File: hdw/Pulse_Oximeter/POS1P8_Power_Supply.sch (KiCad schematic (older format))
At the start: 0 parts

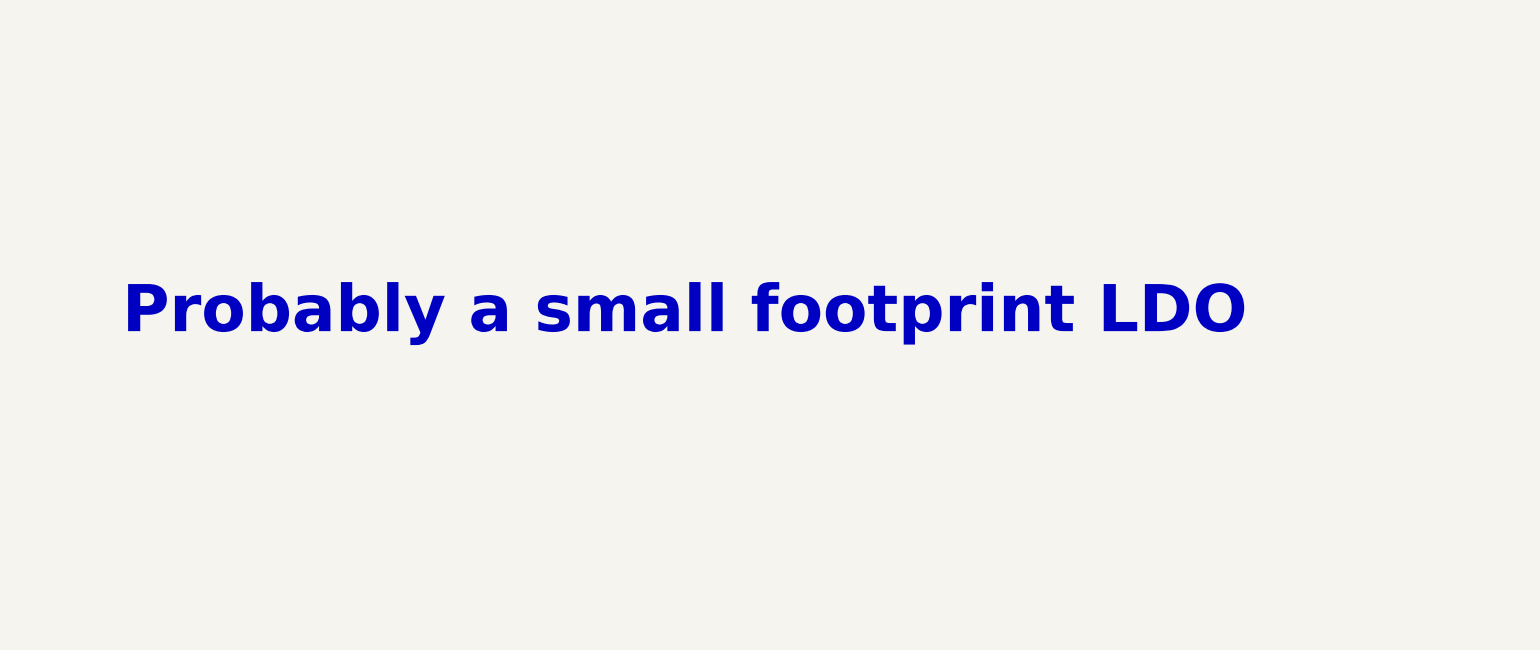
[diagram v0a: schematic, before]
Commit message: Continued schematic development
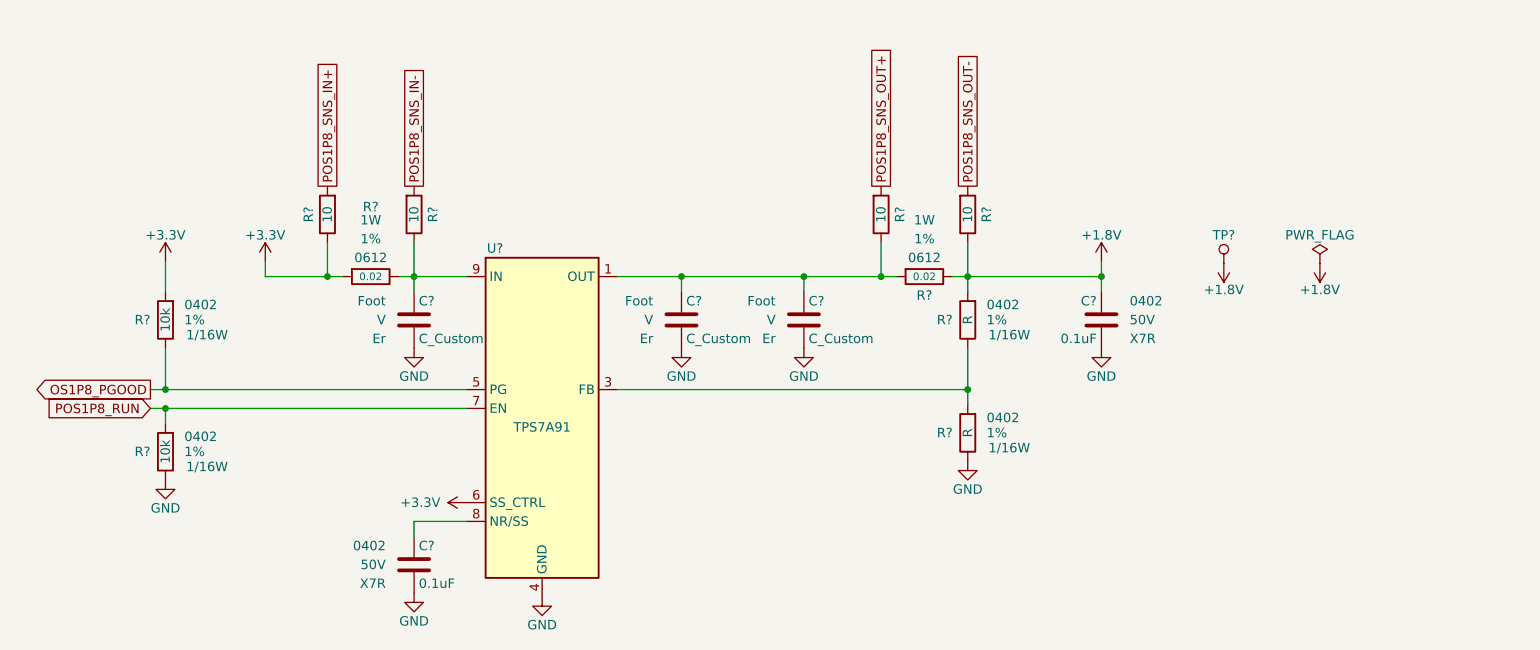
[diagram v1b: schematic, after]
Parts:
- added C? (x2): 0.1uF, Capacitors_SMD:C_0402, symbol Custom_Library:C_Custom
- added C? (x3): C_Custom, symbol Custom_Library:C_Custom
- added R? (x2): 10k, Resistors_SMD:R_0402, symbol Custom_Library:R_Custom
- added R? (x2): 0.02, Resistors_SMD:R_0612, symbol Custom_Library:R_Custom
- added R? (x4): 10, Resistors_SMD:R_0603, symbol Custom_Library:R_Custom
- added R? (x2): R, Resistors_SMD:R_0402, symbol Custom_Library:R_Custom
- added TP?: TP, Custom Footprints Library:Test_Point, symbol Custom_Library:TP
- added U?: TPS7A91, Package_DFN_QFN:Texas_S-PDSO-N10_EP1.2x2mm, symbol Custom_Library:TPS7A91
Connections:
- new net: C?.1, U?.8 (NR/SS)
- new net: C?.1, C?.1, R?.1, R?.2, U?.1 (OUT), U?.2 (OUT)
- new net: C?.1, R?.2, R?.2, U?.10 (IN), U?.9 (IN)
- new net: R?.1, R?.2, U?.3 (FB)
- new net +1.8V: C?.1, R?.1, R?.2, R?.2, TP?.1 (TP)
- new net +3V3: R?.1, R?.1, R?.2, U?.6 (SS_CTRL)
- new net GND: C?.2, C?.2, C?.2, C?.2, C?.2, R?.2, R?.2, U?.11 (GND), U?.4 (GND)
- new net OS1P8_PGOOD: R?.2, U?.5 (PG)
- new net POS1P8_RUN: R?.1, U?.7 (EN)
- new net POS1P8_SNS_IN+: R?.1
- new net POS1P8_SNS_IN-: R?.1
- new net POS1P8_SNS_OUT+: R?.1
- new net POS1P8_SNS_OUT-: R?.1
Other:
- note removed: "Probably a small footprint LDO"
